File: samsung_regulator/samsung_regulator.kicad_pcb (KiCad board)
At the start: 2 copper layers, 9 parts, among them K1 CONN_3

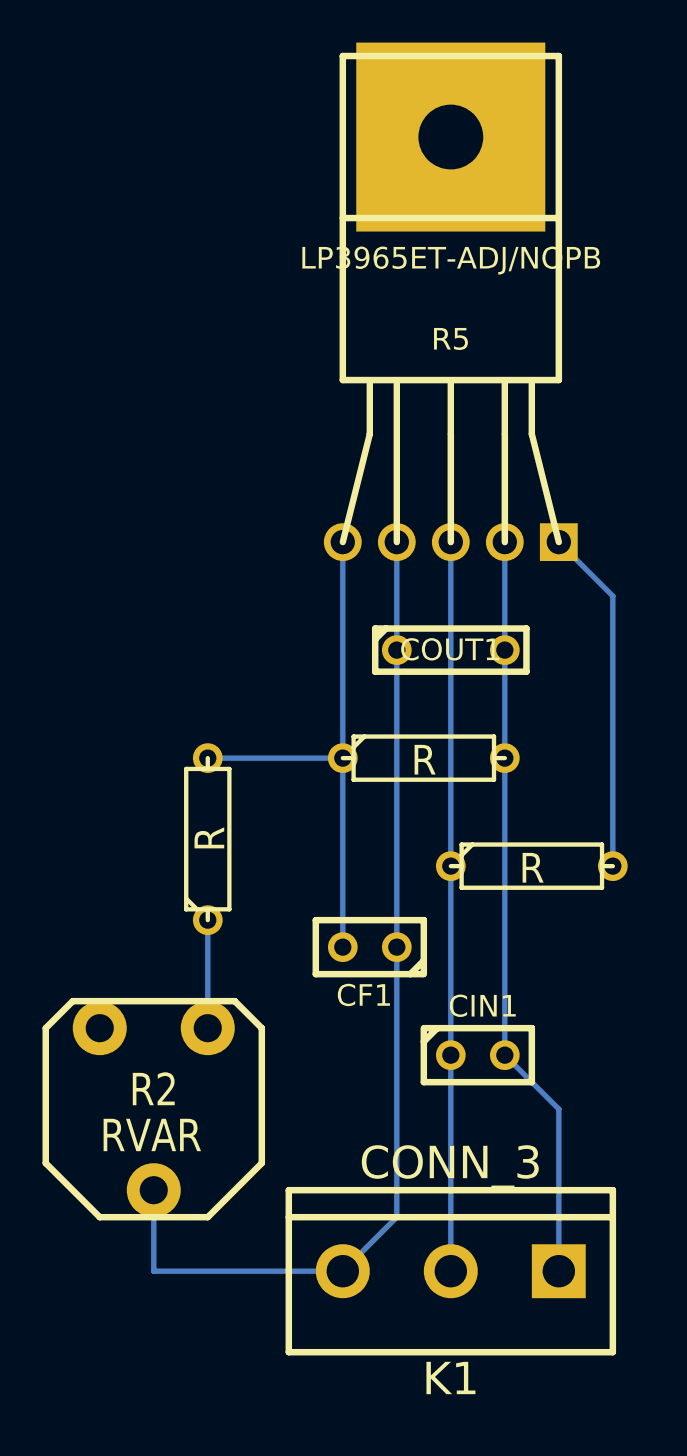
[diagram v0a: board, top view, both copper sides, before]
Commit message: up
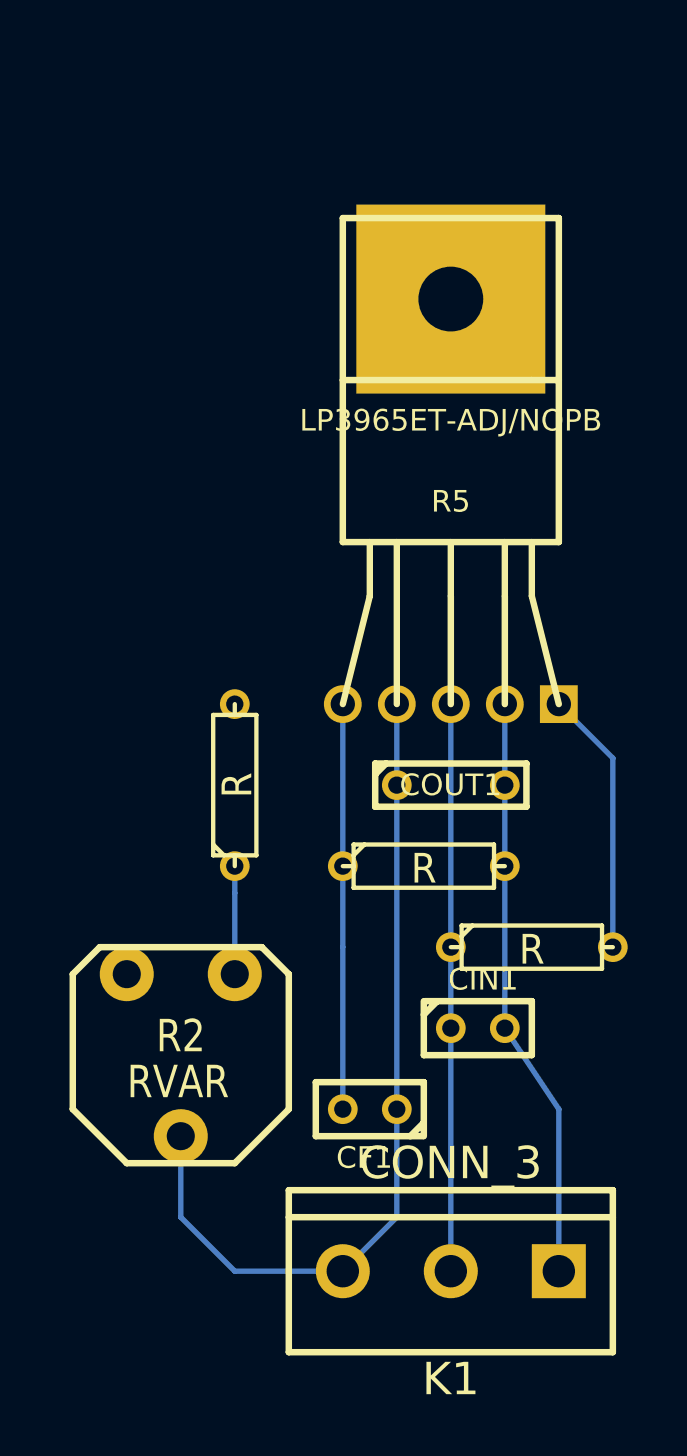
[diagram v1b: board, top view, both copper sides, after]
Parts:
- moved CF1 7.62 mm to (181.6, 90.2)
- moved R5 7.62 mm to (185.4, 68.6)
- moved COUT1 6.35 mm to (185.4, 74.9)
- moved R1 5.08 mm to (184.2, 78.7)
- moved R4 3.81 mm to (189.2, 82.5)
- moved R2 2.84 mm to (172.7, 87.6)
- moved R3 2.84 mm to (175.3, 74.9)
- moved CIN1 1.27 mm to (186.7, 86.4)
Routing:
- net GND: track 35.3 -> 27.4 mm
- net N-000004: track 48.0 -> 40.2 mm
- net N-000006: track 34.3 -> 26.7 mm
- net N-000005: track 25.4 -> 19.0 mm
- net N-000003: track 16.3 -> 12.5 mm
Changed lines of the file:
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@@
   (general
     (links 16)
-    (no_connects 0)
-    (area 162.153599 37.90982 195.371155 104.0384)
+    (no_connects 1)
+    (area 167.233599 45.52982 195.371155 104.0384)
     (thickness 1.6)
     (drawings 0)
-    (tracks 20)
+    (tracks 22)
     (zones 0)
     (modules 9)
@@
   )
   (module TO220-5 (layer F.Cu)
-    (at 185.42 60.96 90)
+    (at 185.42 68.58 90)
     (descr "Transistor TO 220-5")
     (tags "TR TO220 DEV")
@@
   )
   (module R3 (layer F.Cu)
-    (at 184.15 73.66)
+    (at 184.15 78.74)
     (descr "Resitance 3 pas")
     (tags R)
@@
   )
   (module R3 (layer F.Cu)
-    (at 173.99 77.47 90)
+    (at 175.26 74.93 90)
     (descr "Resitance 3 pas")
     (tags R)
@@
   )
   (module R3 (layer F.Cu)
-    (at 189.23 78.74)
+    (at 189.23 82.55)
     (descr "Resitance 3 pas")
     (tags R)
@@
   )
   (module C1 (layer F.Cu)
-    (at 186.69 87.63)
+    (at 186.69 86.36)
     (descr "Condensateur e = 1 pas")
     (tags C)
@@
   )
   (module C1 (layer F.Cu)
-    (at 181.61 82.55 180)
+    (at 181.61 90.17 180)
     (descr "Condensateur e = 1 pas")
     (tags C)
@@
   )
   (module C2 (layer F.Cu)
-    (at 185.42 68.58)
+    (at 185.42 74.93)
     (descr "Condensateur = 2 pas")
     (tags C)
@@
   )
   (module RVAR (layer F.Cu)
-    (at 171.45 90.17 180)
+    (at 172.72 87.63 180)
     (descr "Resistance variable")
     (tags RV)
@@
     )
   )
-  (segment (start 187.96 63.5) (end 187.96 68.58) (width 0.254) (layer B.Cu) (net 1))
-  (segment (start 187.96 68.58) (end 187.96 73.66) (width 0.254) (layer B.Cu) (net 1))
-  (segment (start 187.96 73.66) (end 187.96 87.63) (width 0.254) (layer B.Cu) (net 1))
+  (segment (start 187.96 71.12) (end 187.96 74.93) (width 0.254) (layer B.Cu) (net 1))
+  (segment (start 187.96 74.93) (end 187.96 78.74) (width 0.254) (layer B.Cu) (net 1) (status 10))
+  (segment (start 187.96 78.74) (end 187.96 86.36) (width 0.254) (layer B.Cu) (net 1) (status 10))
   (segment (start 190.5 97.79) (end 190.5 90.17) (width 0.254) (layer B.Cu) (net 1))
-  (segment (start 190.5 90.17) (end 187.96 87.63) (width 0.254) (layer B.Cu) (net 1))
-  (segment (start 173.99 86.36) (end 173.99 81.28) (width 0.254) (layer B.Cu) (net 2) (status 20))
-  (segment (start 193.04 78.74) (end 193.04 66.04) (width 0.254) (layer B.Cu) (net 3))
-  (segment (start 193.04 66.04) (end 190.5 63.5) (width 0.254) (layer B.Cu) (net 3))
-  (segment (start 180.34 97.79) (end 171.45 97.79) (width 0.254) (layer B.Cu) (net 4))
-  (segment (start 171.45 97.79) (end 171.45 93.98) (width 0.254) (layer B.Cu) (net 4) (status 20))
-  (segment (start 182.88 63.5) (end 182.88 68.58) (width 0.254) (layer B.Cu) (net 4))
-  (segment (start 182.88 68.58) (end 182.88 82.55) (width 0.254) (layer B.Cu) (net 4) (status 20))
-  (segment (start 182.88 82.55) (end 182.88 95.25) (width 0.254) (layer B.Cu) (net 4) (status 10))
+  (segment (start 190.5 90.17) (end 187.96 86.36) (width 0.254) (layer B.Cu) (net 1) (status 20))
+  (segment (start 175.26 83.82) (end 175.26 80.01) (width 0.254) (layer B.Cu) (net 2))
+  (segment (start 175.26 80.01) (end 175.26 78.74) (width 0.254) (layer B.Cu) (net 2) (status 20))
+  (segment (start 190.5 71.12) (end 193.04 73.66) (width 0.254) (layer B.Cu) (net 3))
+  (segment (start 193.04 73.66) (end 193.04 82.55) (width 0.254) (layer B.Cu) (net 3))
+  (segment (start 172.72 91.44) (end 172.72 95.25) (width 0.254) (layer B.Cu) (net 4))
+  (segment (start 175.26 97.79) (end 180.34 97.79) (width 0.254) (layer B.Cu) (net 4))
+  (segment (start 172.72 95.25) (end 175.26 97.79) (width 0.254) (layer B.Cu) (net 4))
+  (segment (start 182.88 74.93) (end 182.88 71.12) (width 0.254) (layer B.Cu) (net 4))
+  (segment (start 182.88 74.93) (end 182.88 90.17) (width 0.254) (layer B.Cu) (net 4) (status 10))
+  (segment (start 182.88 90.17) (end 182.88 95.25) (width 0.254) (layer B.Cu) (net 4) (status 10))
   (segment (start 182.88 95.25) (end 180.34 97.79) (width 0.254) (layer B.Cu) (net 4))
-  (segment (start 173.99 73.66) (end 180.34 73.66) (width 0.254) (layer B.Cu) (net 5) (status 10))
-  (segment (start 180.34 73.66) (end 180.34 63.5) (width 0.254) (layer B.Cu) (net 5))
-  (segment (start 180.34 73.66) (end 180.34 82.55) (width 0.254) (layer B.Cu) (net 5) (status 20))
-  (segment (start 185.42 63.5) (end 185.42 78.74) (width 0.254) (layer B.Cu) (net 6))
-  (segment (start 185.42 97.79) (end 185.42 87.63) (width 0.254) (layer B.Cu) (net 6))
-  (segment (start 185.42 87.63) (end 185.42 78.74) (width 0.254) (layer B.Cu) (net 6))
+  (segment (start 180.34 78.74) (end 180.34 71.12) (width 0.254) (layer B.Cu) (net 5))
+  (segment (start 180.34 90.17) (end 180.34 82.55) (width 0.254) (layer B.Cu) (net 5) (status 20))
+  (segment (start 180.34 82.55) (end 180.34 78.74) (width 0.254) (layer B.Cu) (net 5) (status 10))
+  (segment (start 185.42 82.55) (end 185.42 71.12) (width 0.254) (layer B.Cu) (net 6))
+  (segment (start 185.42 97.79) (end 185.42 86.36) (width 0.254) (layer B.Cu) (net 6) (status 20))
+  (segment (start 185.42 86.36) (end 185.42 82.55) (width 0.254) (layer B.Cu) (net 6) (status 10))
 )
